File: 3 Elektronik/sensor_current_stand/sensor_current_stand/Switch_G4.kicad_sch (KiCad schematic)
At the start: 1 part, among them J8 DC37_Plug_MountingHoles

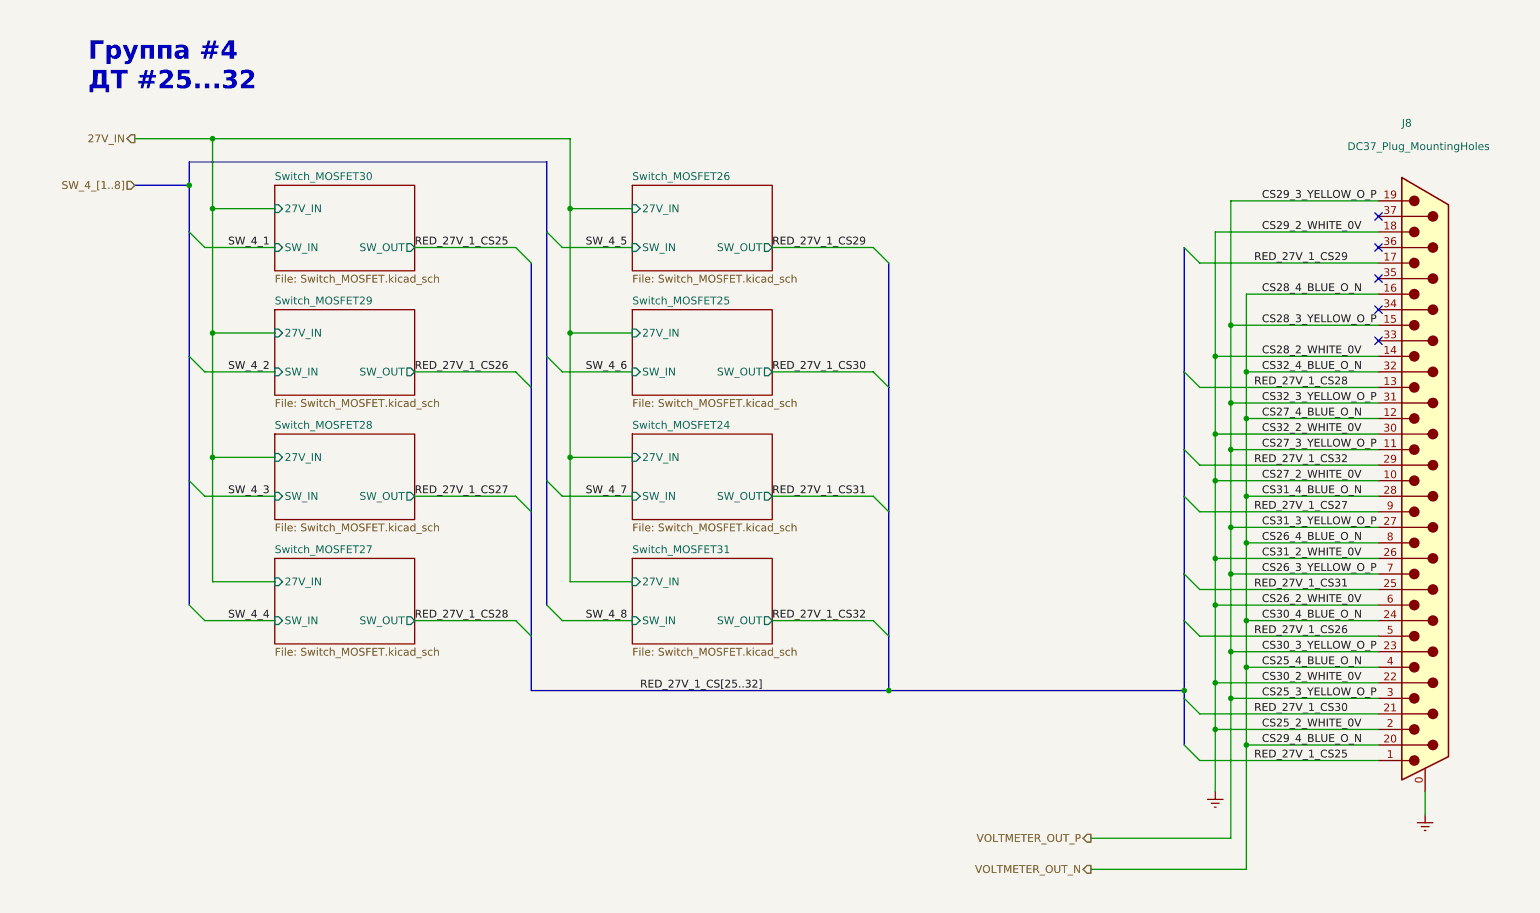
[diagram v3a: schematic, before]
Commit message: Version 2
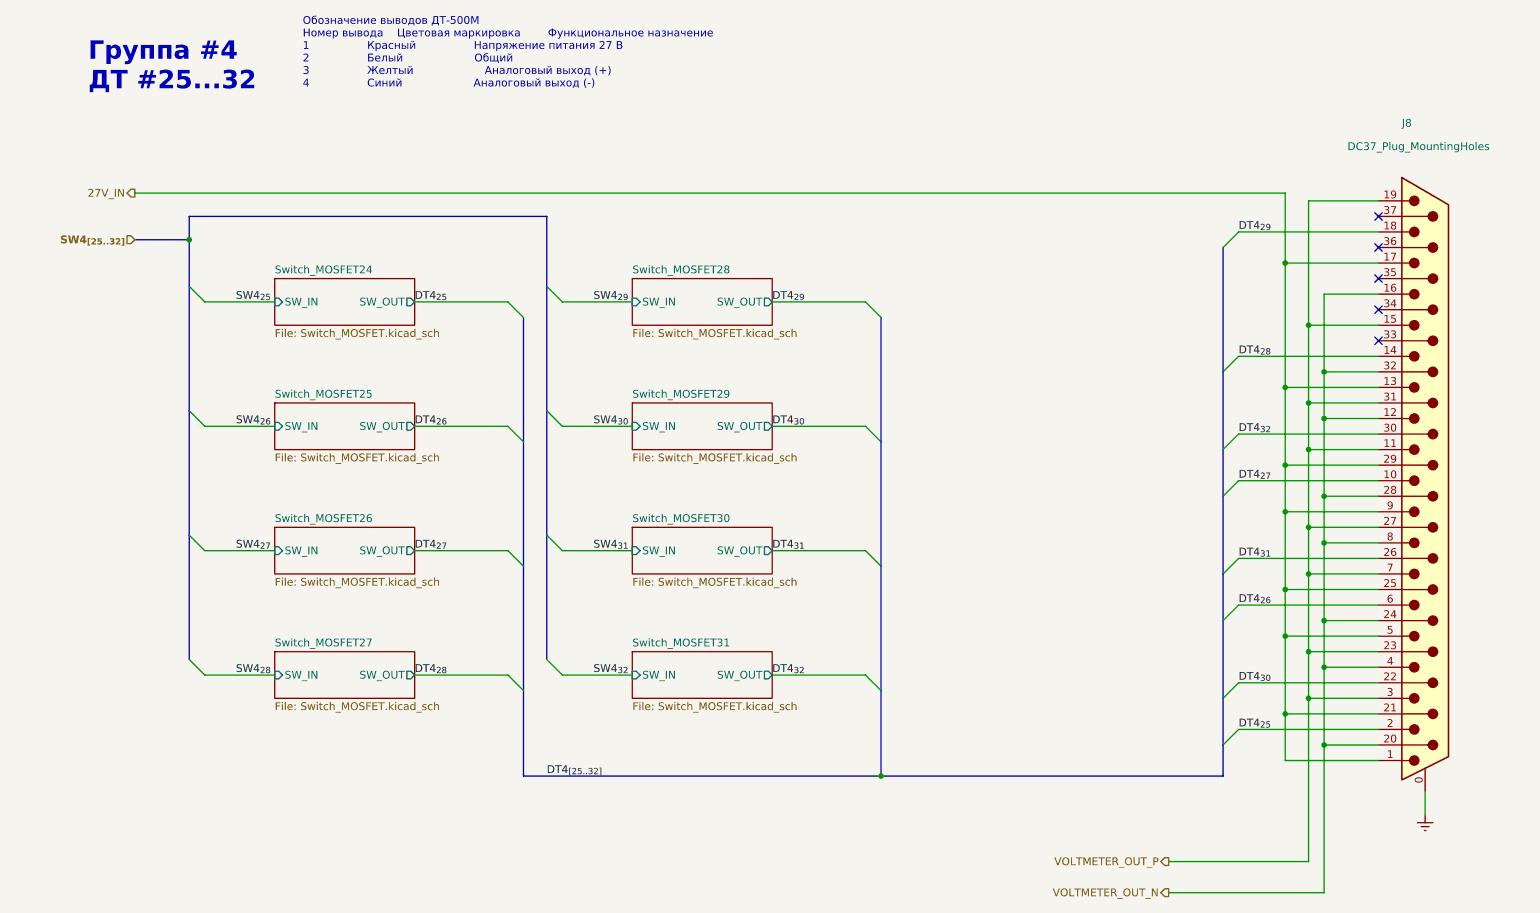
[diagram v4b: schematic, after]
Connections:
- net RED_27V_1_CS25 is gone; now on net 27V_IN: J8.1
- net RED_27V_1_CS26 is gone; now on net 27V_IN: J8.5
- net RED_27V_1_CS27 is gone; now on net 27V_IN: J8.9
- net RED_27V_1_CS28 is gone; now on net 27V_IN: J8.13
- net RED_27V_1_CS29 is gone; now on net 27V_IN: J8.17
- net RED_27V_1_CS30 is gone; now on net 27V_IN: J8.21
- net RED_27V_1_CS31 is gone; now on net 27V_IN: J8.25
- net RED_27V_1_CS32 is gone; now on net 27V_IN: J8.29
- net Earth: no longer J8.10, J8.14, J8.18, J8.2, J8.22, J8.26, J8.30, J8.6
- new net DT4_{25}: J8.2
- new net DT4_{26}: J8.6
- new net DT4_{27}: J8.10
- new net DT4_{28}: J8.14
- new net DT4_{29}: J8.18
- new net DT4_{30}: J8.22
- new net DT4_{31}: J8.26
- new net DT4_{32}: J8.30
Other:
- sheet Switch_MOSFET24 ports: added none; removed 27V_IN
- sheet Switch_MOSFET25 ports: added none; removed 27V_IN
- sheet Switch_MOSFET26 ports: added none; removed 27V_IN
- sheet Switch_MOSFET27 ports: added none; removed 27V_IN
- sheet Switch_MOSFET28 ports: added none; removed 27V_IN
- sheet Switch_MOSFET29 ports: added none; removed 27V_IN
- sheet Switch_MOSFET30 ports: added none; removed 27V_IN
- sheet Switch_MOSFET31 ports: added none; removed 27V_IN
- note added: "Обозначение выводов ДТ-500М Номер вывода Цветовая маркировка Функциональное назначение 1 Красный Напряжение питания 27 В 2 Белый Общий 3 Желтый Аналоговый выход (+) 4 Синий Аналоговый выход (-)"
